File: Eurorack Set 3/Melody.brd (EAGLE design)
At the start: 39.3 x 106.5 mm, 72 parts, among them IC1 LD1117AS33TR, IC2 MCP6004, IC4 7905, Q2 MMBT3904, U1 MKL02Z32VFK4

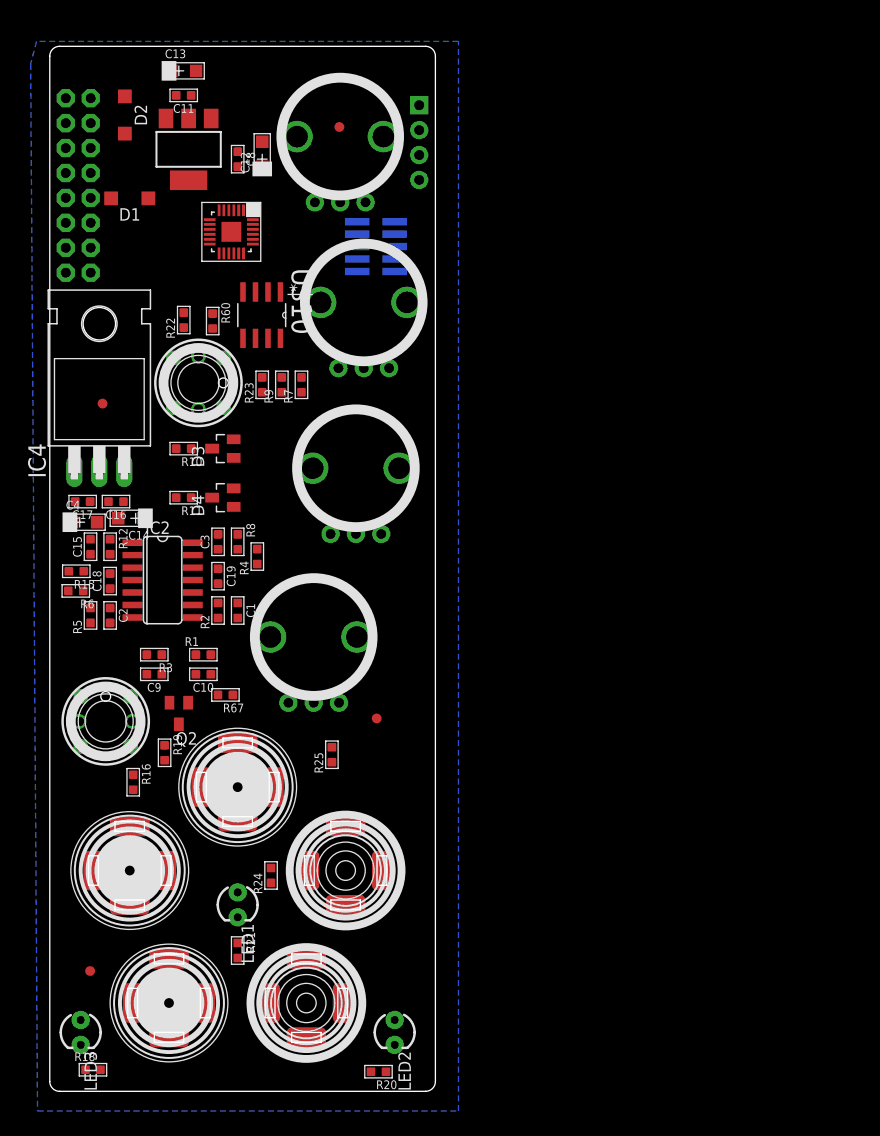
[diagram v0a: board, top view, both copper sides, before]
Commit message: Melody And Screwdriver Updates
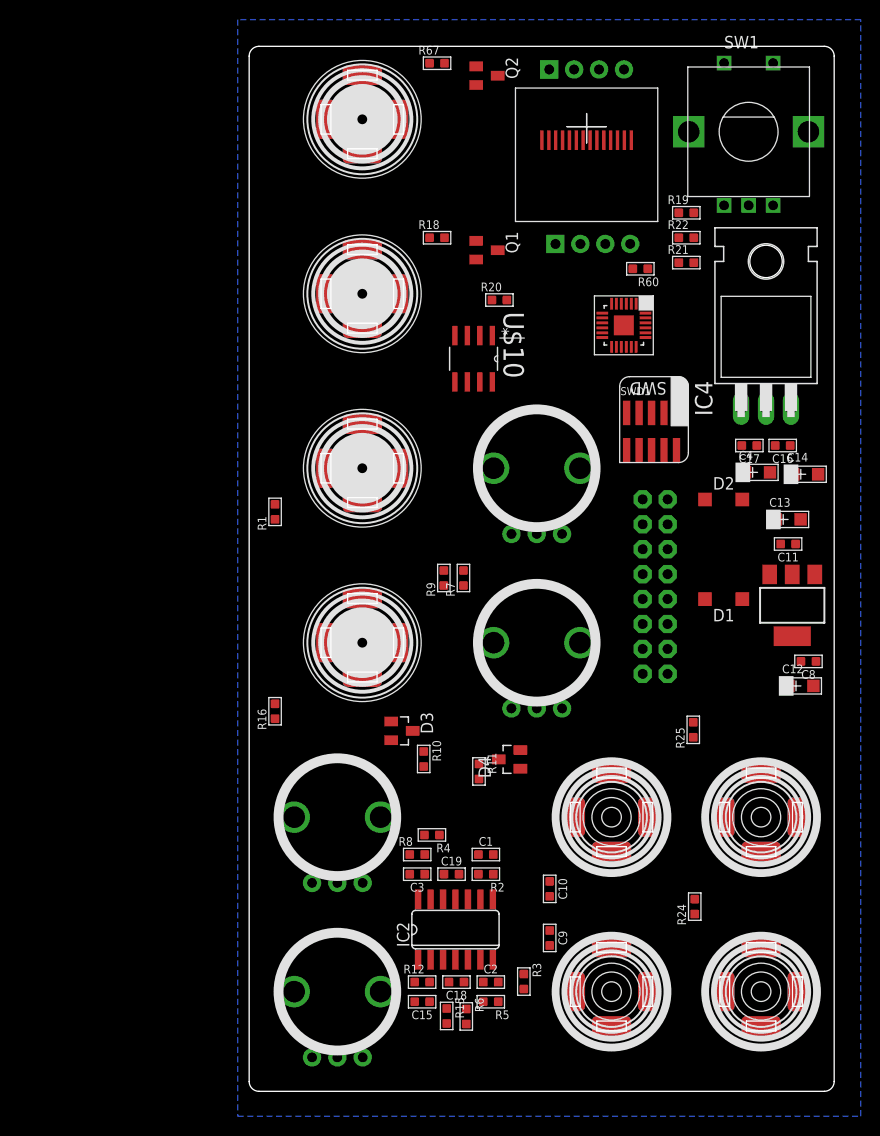
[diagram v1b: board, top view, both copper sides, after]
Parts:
- removed GATE: Gate, EurorackModularParts:3.5MM-JACK-SWITCH-13MM-INPUT
- removed LED1, LED2, LED3: (no value), SparkFun-LED:LED3MM
- removed R23: 10k, OPL:R0603
- removed U$11, U$9: FIDUCIAL, adafruit:FIDUCIAL_1MM
- removed U$3, U$6: SWITCH_W_LED_PB6149L-X-102WHITE, zephod-components:PB6149L
- added CLOCK: Clock, EurorackModularParts:3.5MM-JACK-SWITCH-13MM-INPUT
- added JP2: (no value), SparkFun-Connectors:1X04
- added Q1: MMBT3904, transistor:SOT23-BEC
- added RESET: Reset, EurorackModularParts:3.5MM-JACK-SWITCH-13MM-INPUT
- added SW1: EC12E_SW, switch-alps:ALPS_EC12E_SW
- added U$12: 0.49"OLEDFOLDED, zephod-tft:0.49"-FPC-0.7-14-FOLDED
- R18: value 2k -> 100k
- R19, R22: value 56 -> 33k
- R20: value 2k -> 10k
- R21: value 2k -> 33k
- U$2: value EURORACK_PCB8HP -> EURORACK_PCB12HP; device EurorackModularParts:EURORACK8HPPCB -> EurorackModularParts:EURORACK12HPPCB
- U$4: value FIDUCIAL -> GATE2; device adafruit:FIDUCIAL_1MM -> EurorackModularParts:3.5MM-JACK-SWITCH-13MM-OUTPUT
- U$5: value FIDUCIAL -> GATE1; device adafruit:FIDUCIAL_1MM -> EurorackModularParts:3.5MM-JACK-SWITCH-13MM-OUTPUT
- U$7: value Out 2 -> CV2
- U$8: value Out 1 -> CV1
- moved U$4 92.4 mm to (38.1, 10.2)
- moved R18 91.8 mm to (20.3, 87.0)
- moved R21 83.7 mm to (45.7, 84.5), turned to 0 degrees
- moved R20 79.6 mm to (26.7, 80.6), turned to 0 degrees
- moved C8 77.5 mm to (58.2, 43.8), turned to 180 degrees
- moved C12 77.1 mm to (57.4, 41.3), turned to 0 degrees
- moved IC1 77.1 mm to (56.5, 49.5)
- moved C11 76.7 mm to (56.1, 55.8)
- moved C13 76.7 mm to (56.1, 58.3)
- moved R19 76.5 mm to (45.7, 89.5), turned to 0 degrees
- moved D1 73.0 mm to (49.5, 50.2)
- moved D2 72.5 mm to (49.5, 60.3), turned to 0 degrees
- moved Q2 72.2 mm to (25.4, 103.5), turned to 270 degrees
- moved U$1 71.6 mm to (42.5, 54.0)
- moved R17 70.3 mm to (10.2, 10.2)
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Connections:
- removed net LED1: U$6.LEDPOS, U1.1
- removed net LED2: LED1.A, U1.20
- removed net LED3: LED2.A, U1.14
- removed net LED4: LED3.A, U1.13
- removed net N$1: JP1.3, U1.5
- removed net N$19: R22.1, U$3.LEDNEG
- removed net SW1: U$6.1, U$6.2, U1.2
- removed net SW2: R23.1, U$3.1, U$3.2, U1.17
- removed net SW2LED: R22.2, U1.18
- new net ENC_A: R19.2, SW1.A, U1.5
- new net ENC_B: R21.2, SW1.B, U1.6
- new net ENC_S: R22.2, SW1.E, U1.20
- new net RESET: Q1.C, R20.1, U1.13
- new net SCL: JP1.3, U1.17
- new net SDA: JP1.2, U1.18
- net 3.3V: now also R13.P$3, R14.P$3, R17.P$3, R19.1, R20.2, R21.1, R22.1, R90.P$3; no longer R13.P$1, R14.P$1, R17.P$1, R23.2, R90.P$1, U$3.LEDPOS
- net GND: now also CLOCK.RING@1, CLOCK.RING@2, Q1.E, R13.P$1, R14.P$1, R17.P$1, R90.P$1, RESET.RING@1, RESET.RING@2, SW1.C, SW1.D; no longer GATE.RING@1, GATE.RING@2, R13.P$3, R14.P$3, R17.P$3, R18.2, R19.2, R20.2, R21.2, R90.P$3, U$3.3, U$3.4, U$6.3, U$6.4
- net N$14: now also U1.1; no longer R19.1, U$6.LEDNEG
- net N$15: now also Q1.B, R18.2; no longer LED3.K, R18.1
- net N$16: now also R18.1, RESET.TIP@1, RESET.TIP@2; no longer LED2.K, R20.1
- net N$17: now also U1.2; no longer LED1.K, R21.1
- net N$2: now also U1.14; no longer JP1.2, U1.6
- net N$43: now also CLOCK.TIP@1, CLOCK.TIP@2; no longer GATE.TIP@1, GATE.TIP@2
- net RACK_GATE: now also CLOCK.SWITCH@1, CLOCK.SWITCH@2, RESET.SWITCH@1, RESET.SWITCH@2; no longer GATE.SWITCH@1, GATE.SWITCH@2
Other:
- board size 39.3 x 106.5 mm -> 59.6 x 106.5 mm
